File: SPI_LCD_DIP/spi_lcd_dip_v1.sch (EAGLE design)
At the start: 25 parts

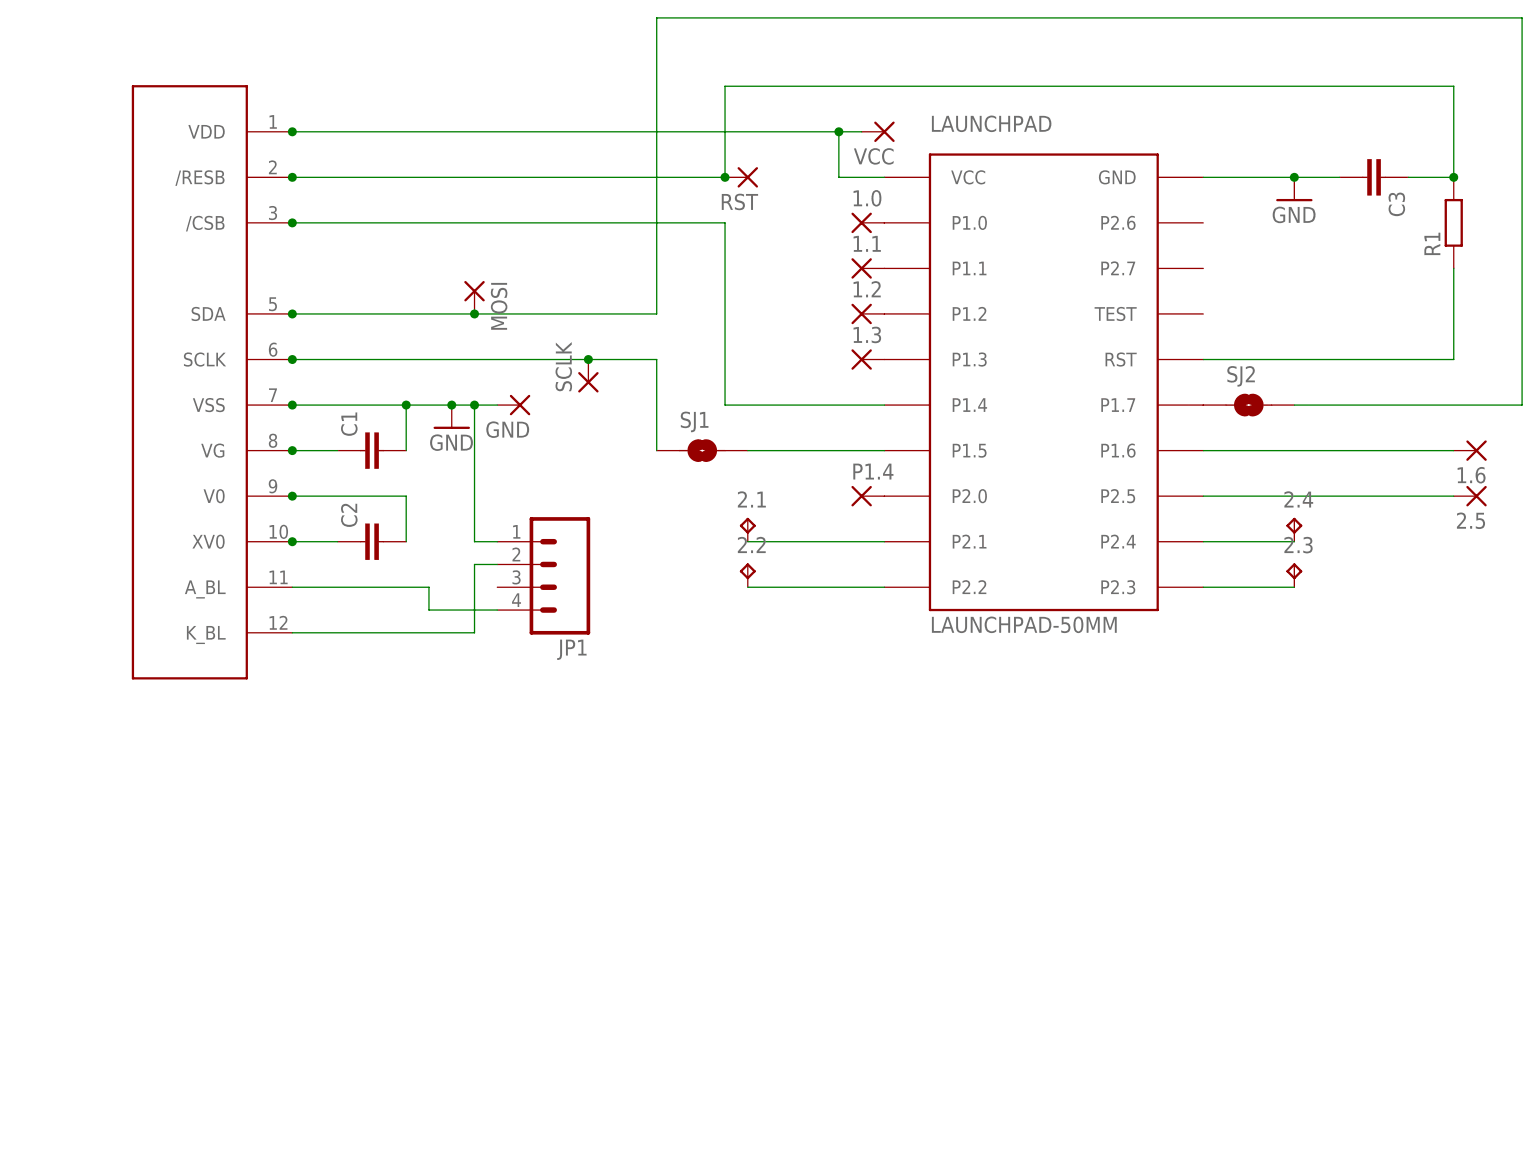
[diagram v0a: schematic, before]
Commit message: Removed wrong, added right
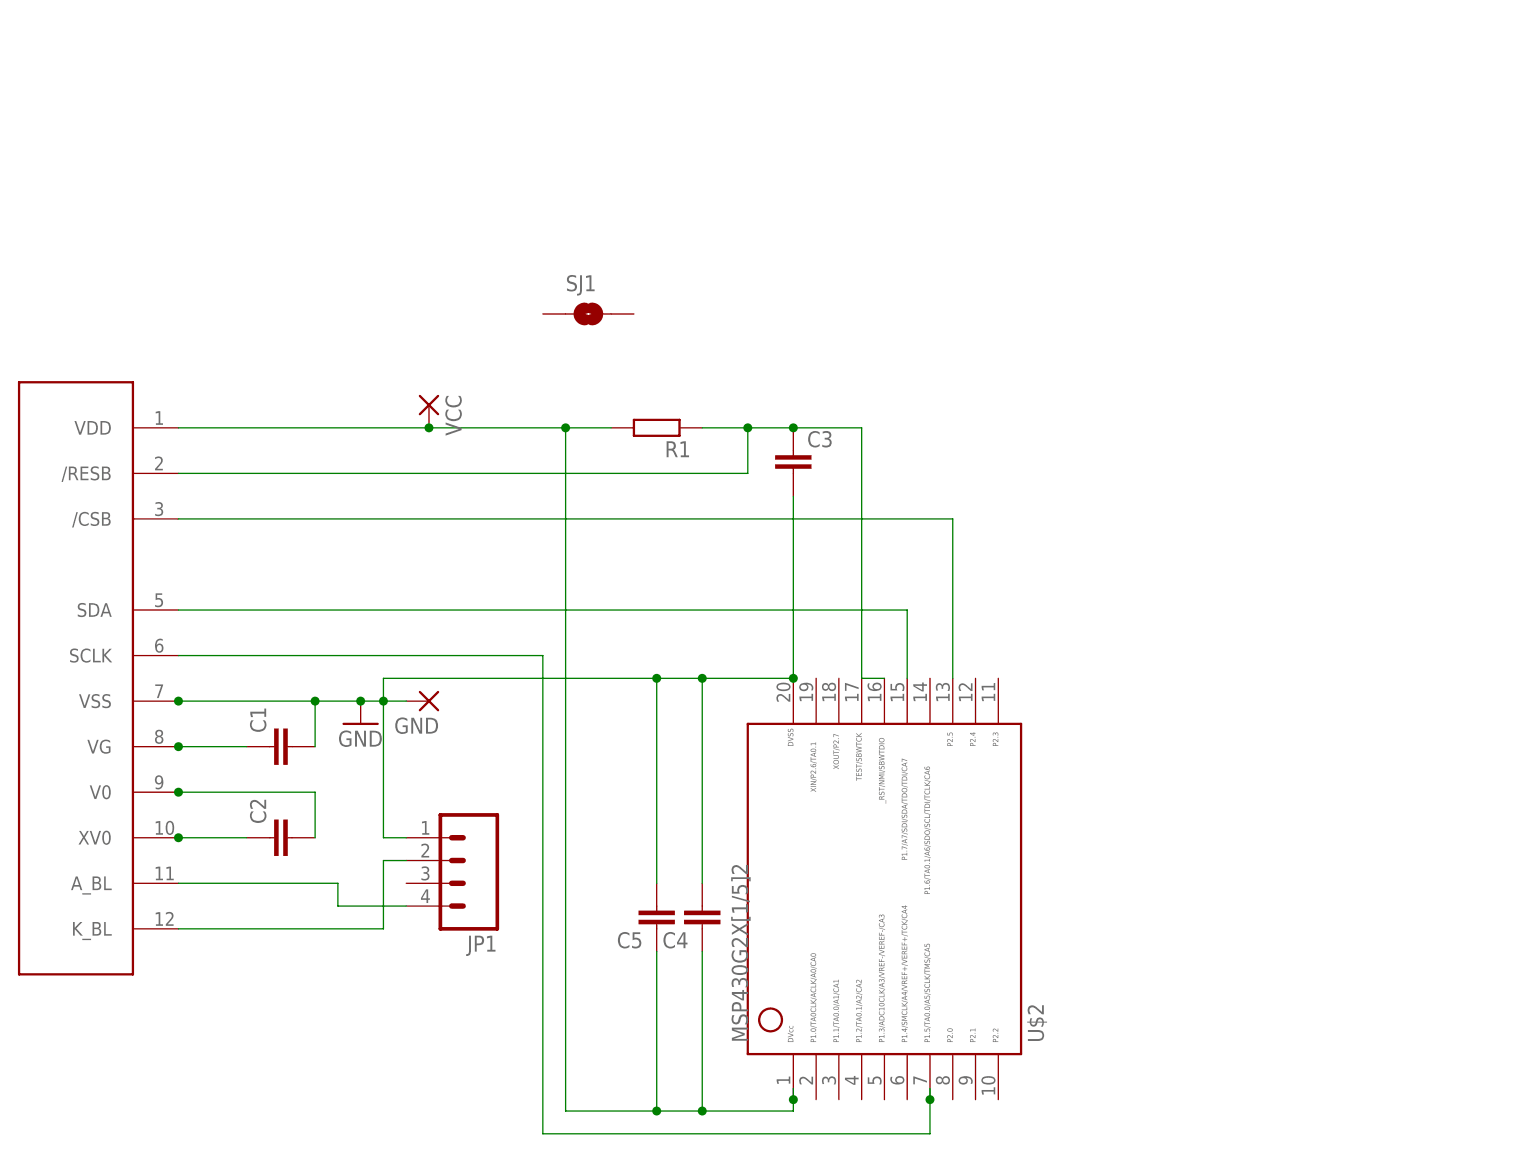
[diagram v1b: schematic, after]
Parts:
- removed 1.0, 1.1, 1.2, 1.3, 1.6, 2.5, MOSI, P1.4, RST, SCLK: (no value), wirepad:2,15/1,0
- removed 2.1, 2.2, 2.3, 2.4: TPTP07R, testpad:TPTP07R
- removed LAUNCHPAD: LAUNCHPAD-50MM, TI_launchpad:LAUNCHPAD-50MM
- removed SJ2: SOLDERJUMPERTRACE, SparkFun-Passives:SOLDERJUMPERTRACE
- added C4, C5: (no value), SparkFun:CAP1206
- added U$2: G2X[1/5]2---N20, TI_MSP430_v16:G2X[1/5]2---N20
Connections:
- removed net N$11: 1.6.P, LAUNCHPAD.P1.6
- removed net N$12: 1.2.P, LAUNCHPAD.P1.2
- removed net N$13: 2.1.TP, LAUNCHPAD.P2.1
- removed net N$14: 2.2.TP, LAUNCHPAD.P2.2
- removed net N$15: 2.4.TP, LAUNCHPAD.P2.4
- removed net N$16: 2.3.TP, LAUNCHPAD.P2.3
- removed net N$17: 1.3.P, LAUNCHPAD.P1.3
- removed net N$18: LAUNCHPAD.P2.0, P1.4.P
- removed net N$19: 1.1.P, LAUNCHPAD.P1.1
- removed net N$20: LAUNCHPAD.P1.7, SJ2.1
- removed net N$21: LAUNCHPAD.P1.5, SJ1.2
- removed net N$4: 2.5.P, LAUNCHPAD.P2.5
- removed net N$7: SCLK.P, SJ1.1, U$1.SCLK
- removed net VDD: LAUNCHPAD.VCC, U$1.VDD, VCC.P
- net GND: now also C4.2, C5.2, U$2.20; no longer LAUNCHPAD.GND
- net N$10: now also U$1.SCLK, U$2.7; no longer LAUNCHPAD.RST, R1.1
- net N$5: now also R1.1, U$2.16; no longer R1.2, RST.P
- net N$6: now also C4.1, C5.1, R1.2, U$1.VDD, U$2.1, VCC.P; no longer 1.0.P, LAUNCHPAD.P1.0
- net N$8: now also U$2.15; no longer MOSI.P, SJ2.2
- net N$9: now also U$2.13; no longer LAUNCHPAD.P1.4
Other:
- moved on the sheet: C1, C2, C3, GND, JP1, R1, SJ1, VCC
